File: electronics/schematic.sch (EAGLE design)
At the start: 14 parts, among them Q1 MC-405, Q3 SST201

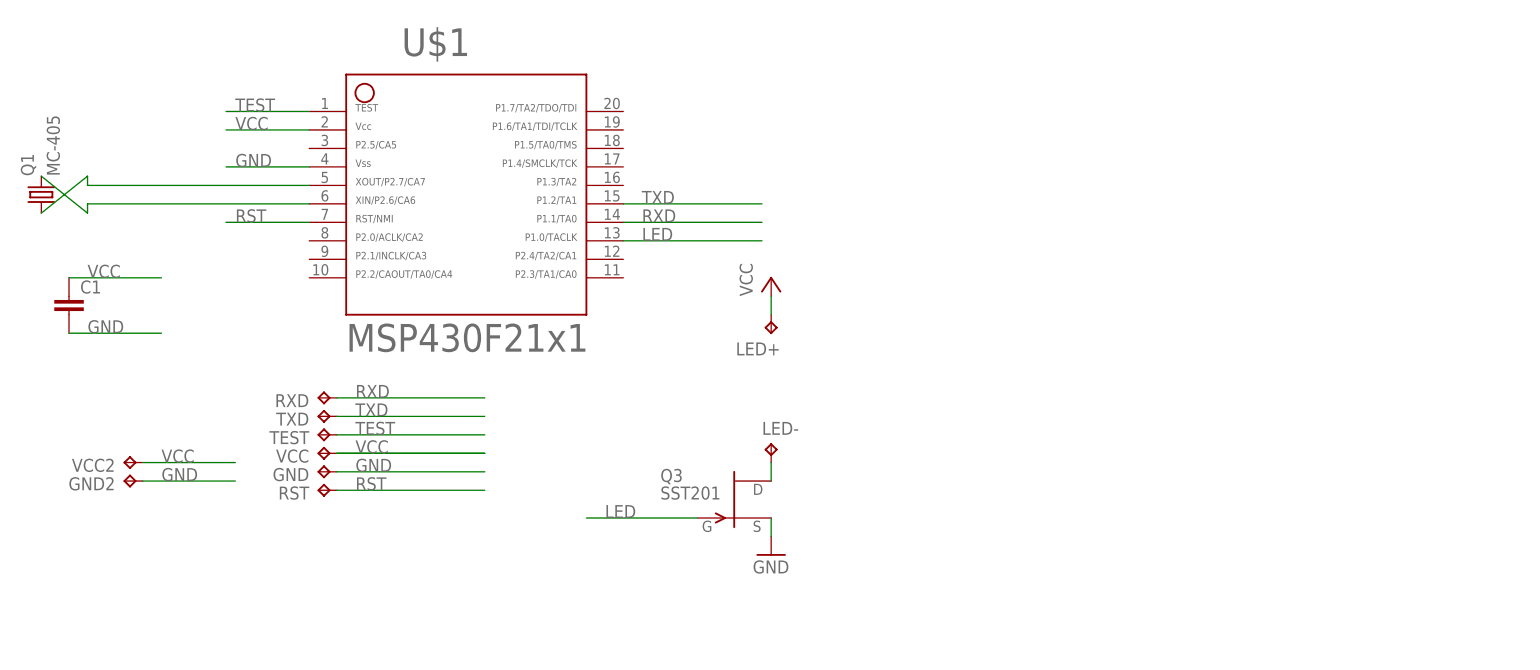
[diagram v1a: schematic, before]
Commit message: RC0. Actual MOSTFET. Added sync pulse. Included LEDs
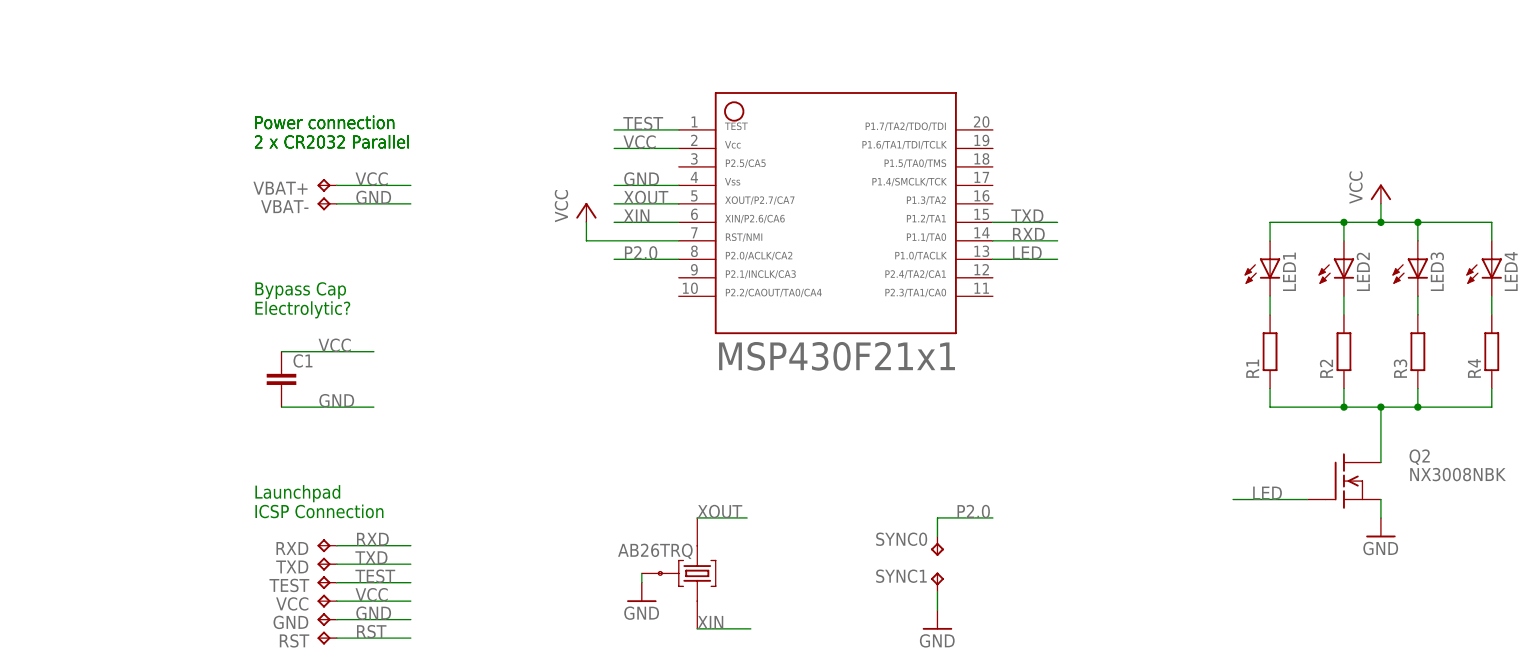
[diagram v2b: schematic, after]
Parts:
- removed GND2, LED+, LED-, VCC2: TPTP15R, testpad:TPTP15R
- removed Q1: MC-405, ROB:MC-405
- removed Q3: SST201, transistor-fet:SST201
- added LED1, LED2, LED3, LED4: (no value), led:LEDCHIP-LED0805
- added Q2: NX3008NBK, playafly:NX3008NBK
- added R1, R2, R3, R4: (no value), resistor:R-EU_M0805
- added SYNC0, SYNC1, VBAT+, VBAT-: TPTP15R, testpad:TPTP15R
- added U$2: AB26TRQ, playafly:AB26TRQ
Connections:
- removed net N$1: Q1.1, U$1.5
- removed net N$2: Q1.2, U$1.6
- new net N$5: LED2.C, R2.2
- new net N$6: LED3.C, R3.2
- new net N$7: LED4.C, R4.2
- new net N$8: Q2.D, R1.1, R2.1, R3.1, R4.1
- new net P2.0: SYNC0.TP, U$1.8
- new net XIN: U$1.6, U$2.1
- new net XOUT: U$1.5, U$2.2
- net GND: now also Q2.S, SYNC1.TP, U$2.3, VBAT-.TP; no longer GND2.TP, Q3.S
- net LED: now also Q2.G; no longer Q3.G
- net N$4: now also LED1.C, R1.2; no longer LED-.TP, Q3.D
- net RST: no longer U$1.7
- net VCC: now also LED1.A, LED2.A, LED3.A, LED4.A, U$1.7, VBAT+.TP; no longer LED+.TP, VCC2.TP
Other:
- note added: "Bypass Cap Electrolytic?"
- note added: "Launchpad ICSP Connection"
- note added: "Power connection 2 x CR2032 Parallel"
- moved on the sheet: C1, GND, RST, RXD, TEST, TXD, VCC
